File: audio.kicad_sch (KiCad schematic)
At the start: 16 parts, among them J1 HEADER_3, U9 PCM5102A, X1 STEREO_AUDIO_JACK

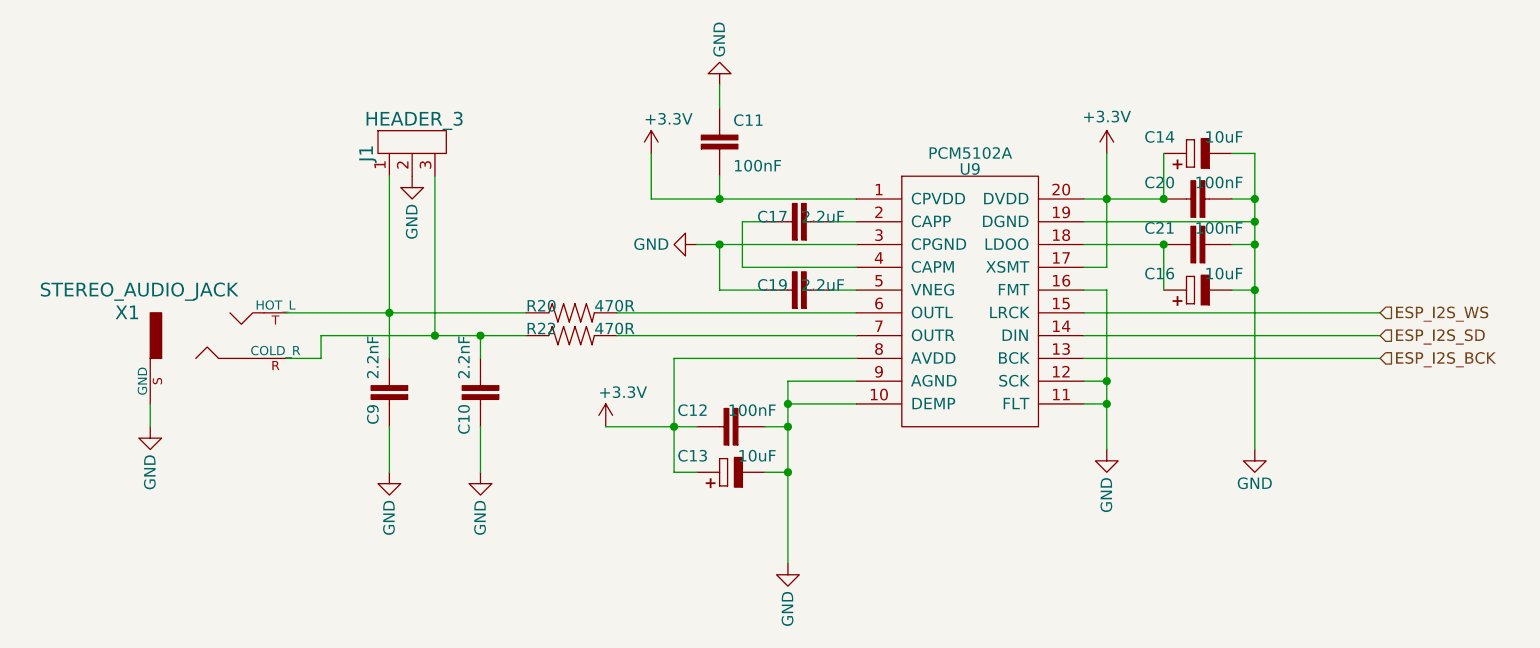
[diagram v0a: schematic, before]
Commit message: 1st production and BOM
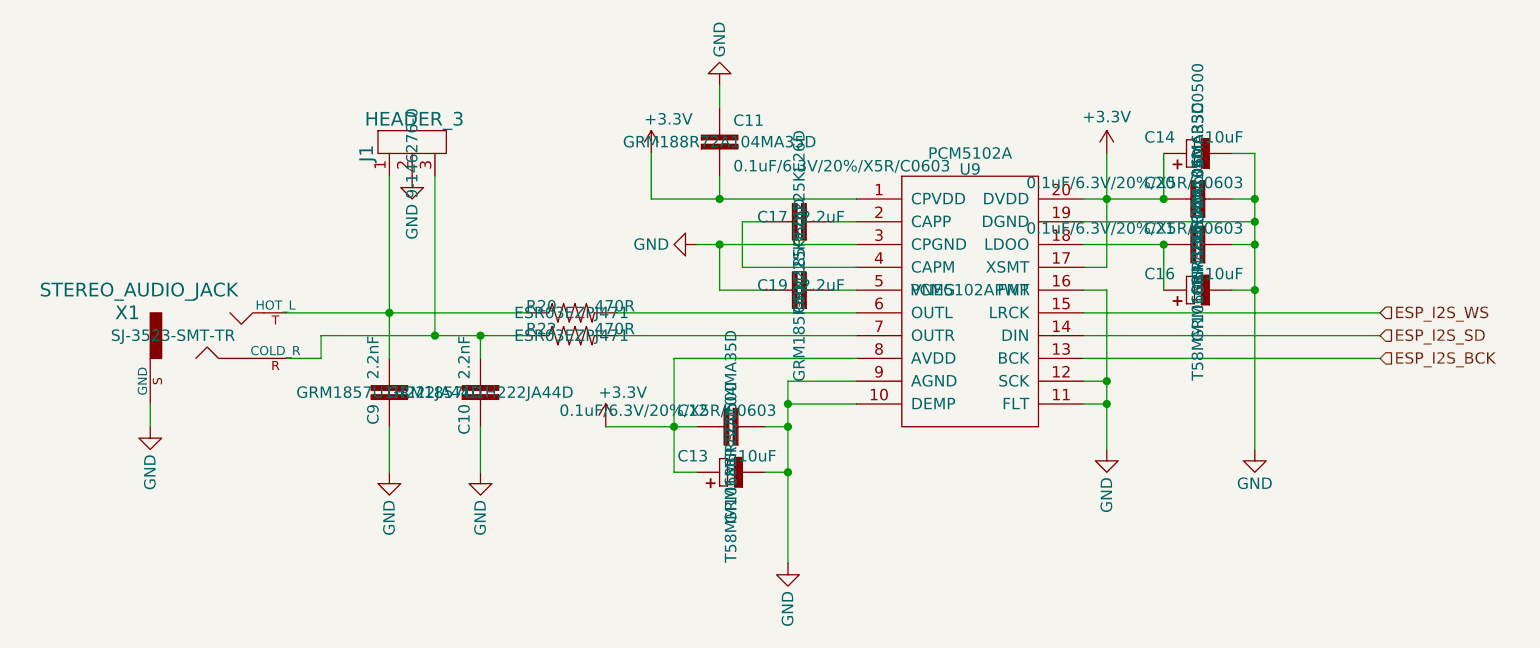
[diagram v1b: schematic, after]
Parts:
- C10, C9: MfgNumber (none) -> GRM1857U1H222JA44D
- C11, C12, C20, C21: value 100nF -> 0.1uF/6.3V/20%/X5R/C0603; MfgNumber (none) -> GRM188R72A104MA35D
- C13, C14, C16: MfgNumber (none) -> T58MM106M6R3C0500
- C17, C19: MfgNumber (none) -> GRM185R60J225KE26D
- J1: MfgNumber (none) -> 9-146276-0
- R20, R22: MfgNumber (none) -> ESR03EZPJ471
- U9: MfgNumber (none) -> PCM5102APWR
- X1: MfgNumber (none) -> SJ-3523-SMT-TR
